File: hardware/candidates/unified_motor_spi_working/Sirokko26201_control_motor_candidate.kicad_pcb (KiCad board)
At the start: 2 copper layers, 180 x 170 mm, 112 parts, among them J1 DEVKITC1_J1, J10 TC_K_EXHAUST_T+_T-, J102 MOTOR_24V_HIGH_SPEED; 125W_HE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, J11 TC_K_AIR_T+_T-, J12 ROOM_DS18B20_HARNESS, J13 24V_LOGIC_INPUT_ONLY__DRAFT_N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, J22 PANEL_DRY_CONTACTS_3V3, J23 LOCAL_BUTTONS_3V3__SET_UP_DOW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, J24 RESET_HW_SPDT_BBM_3V3, J25 THERMAL_AND_HW_ENABLE_3V3_ONLY, J26 TFT_GMT020-02-7P_ST7789V_7P_S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, J3 DEVKITC1_J3, Q101 IRFB4110PBF (100V; RDS(on) @ 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, U1 TPS3431SDRBR, U10 MAX31856MUD+, U101 LM5013DDAR, U2 SN74HCS74D, U3 SN74HCS14D, U4 SN74HCS30D, U5 SN74HCS30D, U6 SN74HCS11D, U7 TPS3839G33DBZR, U8 SN74LVC1G14DBVR, U9 MAX31856MUD+, U9001 LTC7001IMSE#PBF; MSOP-10 EP, U9002 INA240A1ID, U9003 LMV331M5X/NOPB, U9004 SN74LVC1G32DBVR, U9005 SN74LVC1G08DBVR, U9006 SN74LVC1G08DBVR, U9007 LM317HVT/NOPB TO-220; TJ 0…12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

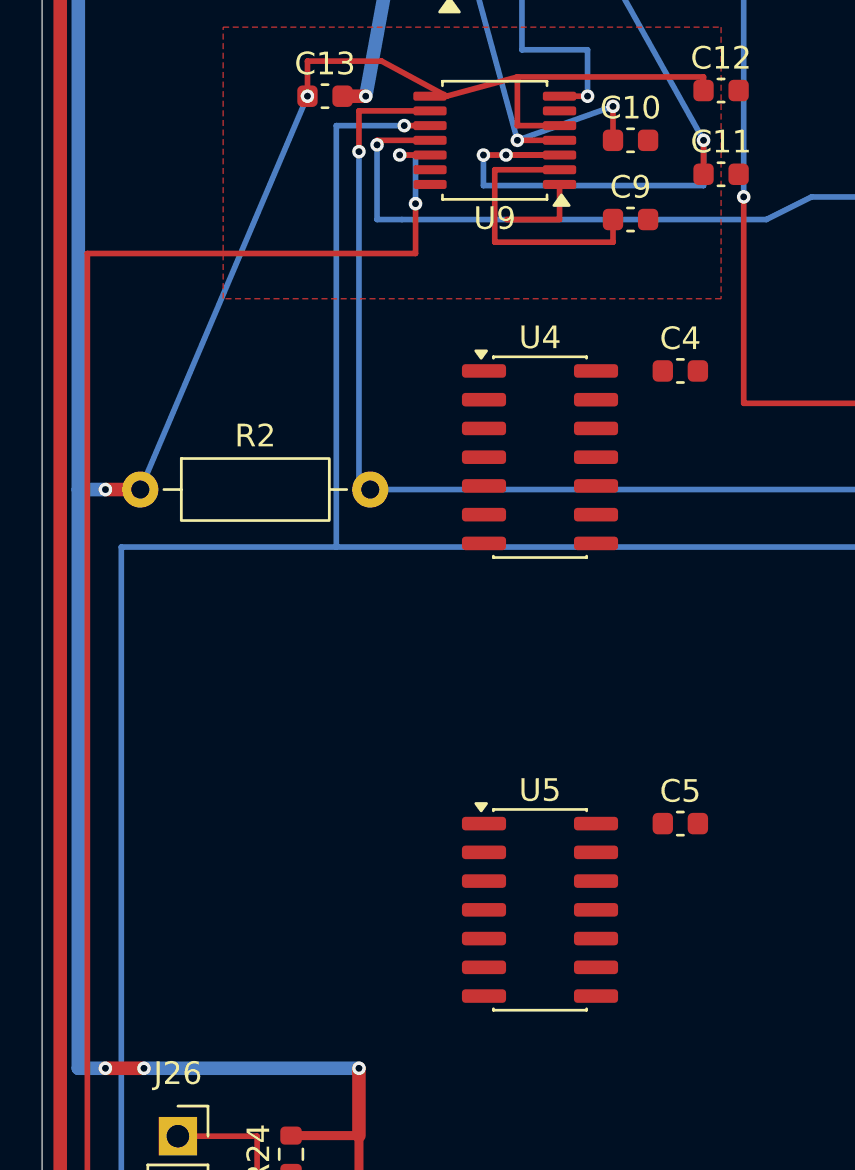
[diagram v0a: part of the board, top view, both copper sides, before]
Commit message: hardware: WIP publish U4/U5 logic supply routing 283/72
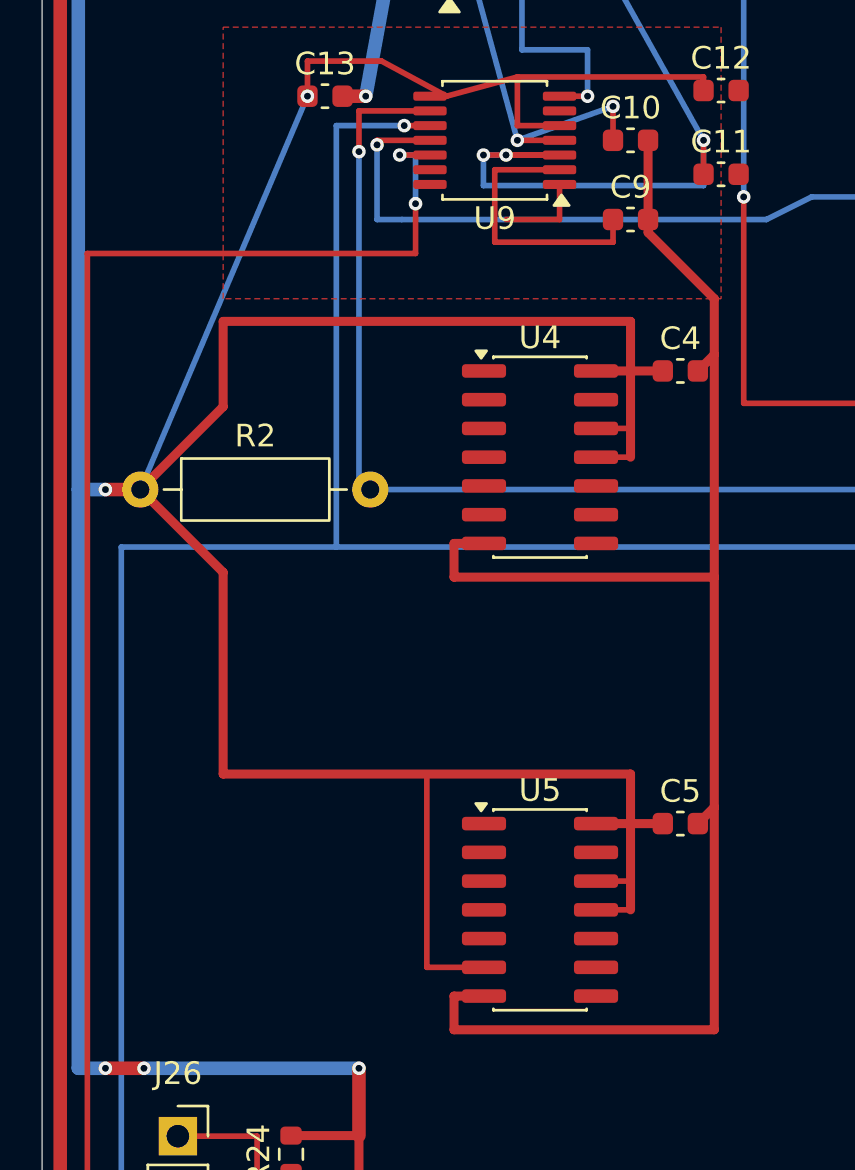
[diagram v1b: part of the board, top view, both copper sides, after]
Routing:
- net /+3V3: track 291.3 -> 385.4 mm
- net /GND: track 500.0 -> 571.2 mm
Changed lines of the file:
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@@
+	)
+	(segment
+		(start 36 61.19)
+		(end 36 65)
+		(width 0.4)
+		(layer "F.Cu")
+		(net "/+3V3")
+	)
+	(segment
+		(start 36 59)
+		(end 36 61.19)
+		(width 0.4)
+		(layer "F.Cu")
+		(net "/+3V3")
 	)
 	(segment
@@
 	)
 	(segment
+		(start 34.475 41.19)
+		(end 37.425 41.19)
+		(width 0.4)
+		(layer "F.Cu")
+		(net "/+3V3")
+	)
+	(segment
 		(start 62.1 31.65)
 		(end 62.1 36.5)
@@
 	)
 	(segment
+		(start 27 59)
+		(end 27 67.54)
+		(width 0.25)
+		(layer "F.Cu")
+		(net "/+3V3")
+	)
+	(segment
 		(start 31 30.35)
 		(end 31 28.2)
@@
 	)
 	(segment
+		(start 18 42.77)
+		(end 18 39)
+		(width 0.4)
+		(layer "F.Cu")
+		(net "/+3V3")
+	)
+	(segment
+		(start 34.475 63.73)
+		(end 36 63.73)
+		(width 0.25)
+		(layer "F.Cu")
+		(net "/+3V3")
+	)
+	(segment
+		(start 14.34 46.43)
+		(end 18 50.09)
+		(width 0.4)
+		(layer "F.Cu")
+		(net "/+3V3")
+	)
+	(segment
 		(start 55.225 36.5)
 		(end 55.225 35.5)
@@
 	)
 	(segment
+		(start 18 50.09)
+		(end 18 59)
+		(width 0.4)
+		(layer "F.Cu")
+		(net "/+3V3")
+	)
+	(segment
 		(start 31 28.2)
 		(end 39.225 28.2)
@@
 	)
 	(segment
+		(start 34.475 43.73)
+		(end 36 43.73)
+		(width 0.25)
+		(layer "F.Cu")
+		(net "/+3V3")
+	)
+	(segment
 		(start 73.225 36.5)
 		(end 73.225 34.8)
@@
 	)
 	(segment
+		(start 14.34 46.43)
+		(end 18 42.77)
+		(width 0.4)
+		(layer "F.Cu")
+		(net "/+3V3")
+	)
+	(segment
+		(start 27 67.54)
+		(end 29.525 67.54)
+		(width 0.25)
+		(layer "F.Cu")
+		(net "/+3V3")
+	)
+	(segment
 		(start 105.86 30.5)
 		(end 105.86 35)
@@
 	)
 	(segment
+		(start 36 41.19)
+		(end 36 45)
+		(width 0.4)
+		(layer "F.Cu")
+		(net "/+3V3")
+	)
+	(segment
+		(start 34.475 65)
+		(end 36 65)
+		(width 0.25)
+		(layer "F.Cu")
+		(net "/+3V3")
+	)
+	(segment
+		(start 34.475 61.19)
+		(end 37.425 61.19)
+		(width 0.4)
+		(layer "F.Cu")
+		(net "/+3V3")
+	)
+	(segment
 		(start 14.5 72)
 		(end 12.8 72)
@@
 	)
 	(segment
+		(start 36 39)
+		(end 36 41.19)
+		(width 0.4)
+		(layer "F.Cu")
+		(net "/+3V3")
+	)
+	(segment
+		(start 18 59)
+		(end 36 59)
+		(width 0.4)
+		(layer "F.Cu")
+		(net "/+3V3")
+	)
+	(segment
 		(start 64.4 31.65)
 		(end 62.5 31.65)
@@
 	)
 	(segment
+		(start 34.475 45)
+		(end 36 45)
+		(width 0.25)
+		(layer "F.Cu")
+		(net "/+3V3")
+	)
+	(segment
 		(start 62.5 36.5)
 		(end 73.225 36.5)
 		(width 0.25)
+		(layer "F.Cu")
+		(net "/+3V3")
+	)
+	(segment
+		(start 18 39)
+		(end 36 39)
+		(width 0.4)
 		(layer "F.Cu")
 		(net "/+3V3")
@@
 	)
 	(segment
+		(start 38.975 61.19)
+		(end 39.7 60.465)
+		(width 0.4)
+		(layer "F.Cu")
+		(net "/GND")
+	)
+	(segment
 		(start 10.8 13.5)
 		(end 83 13.5)
 		(width 0.6)
+		(layer "F.Cu")
+		(net "/GND")
+	)
+	(segment
+		(start 39.7 50.3)
+		(end 39.7 40.465)
+		(width 0.4)
+		(layer "F.Cu")
+		(net "/GND")
+	)
+	(segment
+		(start 29.525 48.81)
+		(end 28.2 48.81)
+		(width 0.4)
 		(layer "F.Cu")
 		(net "/GND")
@@
 	)
 	(segment
+		(start 28.2 70.3)
+		(end 39.7 70.3)
+		(width 0.4)
+		(layer "F.Cu")
+		(net "/GND")
+	)
+	(segment
 		(start 121.975 46.5)
 		(end 123.5 46.5)
@@
 	)
 	(segment
+		(start 39.7 38)
+		(end 36.775 35.075)
+		(width 0.4)
+		(layer "F.Cu")
+		(net "/GND")
+	)
+	(segment
 		(start 121.975 52.5)
 		(end 123.5 52.5)
@@
 	)
 	(segment
+		(start 28.2 68.81)
+		(end 28.2 70.3)
+		(width 0.4)
+		(layer "F.Cu")
+		(net "/GND")
+	)
+	(segment
+		(start 29.525 68.81)
+		(end 28.2 68.81)
+		(width 0.4)
+		(layer "F.Cu")
+		(net "/GND")
+	)
+	(segment
 		(start 168 43.525)
 		(end 173 43.525)
@@
 	)
 	(segment
+		(start 39.7 70.3)
+		(end 39.7 60.465)
+		(width 0.4)
+		(layer "F.Cu")
+		(net "/GND")
+	)
+	(segment
 		(start 121.975 57.5)
 		(end 123.5 57.5)
@@
 	)
 	(segment
+		(start 28.2 48.81)
+		(end 28.2 50.3)
+		(width 0.4)
+		(layer "F.Cu")
+		(net "/GND")
+	)
+	(segment
 		(start 125.3 48.095)
 		(end 128 48.095)
@@
 	)
 	(segment
+		(start 38.975 41.19)
+		(end 39.7 40.465)
+		(width 0.4)
+		(layer "F.Cu")
+		(net "/GND")
+	)
+	(segment
 		(start 16 90.24)
 		(end 10.8 90.24)
@@
 		(end 83 22)
 		(width 0.6)
+		(layer "F.Cu")
+		(net "/GND")
+	)
+	(segment
+		(start 39.7 60.465)
+		(end 39.7 50.3)
+		(width 0.4)
 		(layer "F.Cu")
 		(net "/GND")
@@
 	)
 	(segment
+		(start 28.2 50.3)
+		(end 39.7 50.3)
+		(width 0.4)
+		(layer "F.Cu")
+		(net "/GND")
+	)
+	(segment
 		(start 121.5 61.175)
 		(end 122.7 61.175)
@@
 		(layer "F.Cu")
 		(net "/GND")
+	)
+	(segment
+		(start 36.775 35.075)
+		(end 36.775 31)
+		(width 0.4)
+		(layer "F.Cu")
+		(net "/GND")
+	)
+	(segment
+		(start 39.7 40.465)
+		(end 39.7 38)
+		(width 0.4)
+		(layer "F.Cu")
+		(net "/GND")
